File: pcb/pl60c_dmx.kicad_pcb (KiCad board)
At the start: 2 copper layers, 80 x 54 mm, 39 parts, among them J1 USB-C 16P, J2 XLR-5 female (DMX OUT), J3 DMX pigtail, J4 EXPANSION, J5 UART0, Q1 S8050, SW1 RESET, SW2 BOOT, SW3 USER, U1 ESP32-S3-WROOM-1-N16R8, U2 AMS1117-3.3, U3 SP3485EN, U4 USBLC6-2SC6

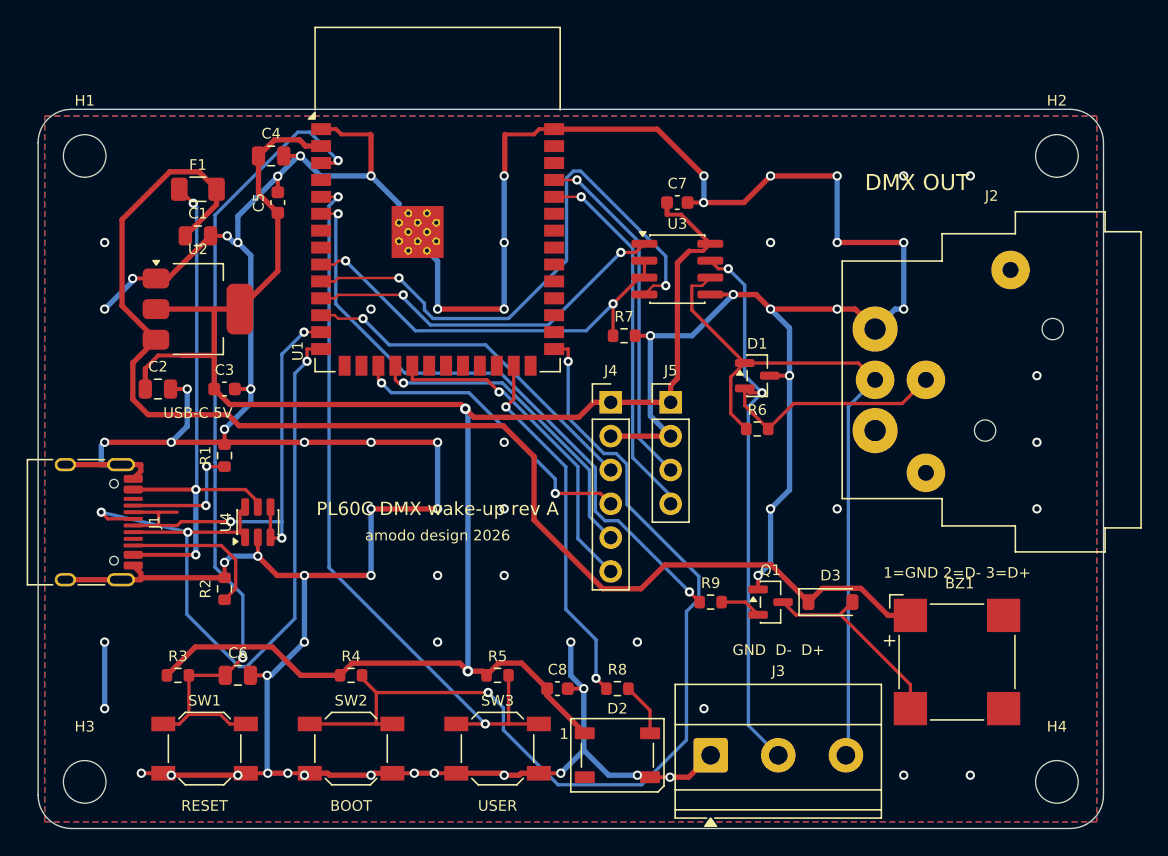
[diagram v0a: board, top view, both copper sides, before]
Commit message: auto: 2026-09-02 13:18:56
Co-Authored-By: Claude Fable 5.1 <noreply@anthropic.com>
Claude-Session: https://claude.ai/code/session_01WsrVZb94LwbHVAmBvsSTfn
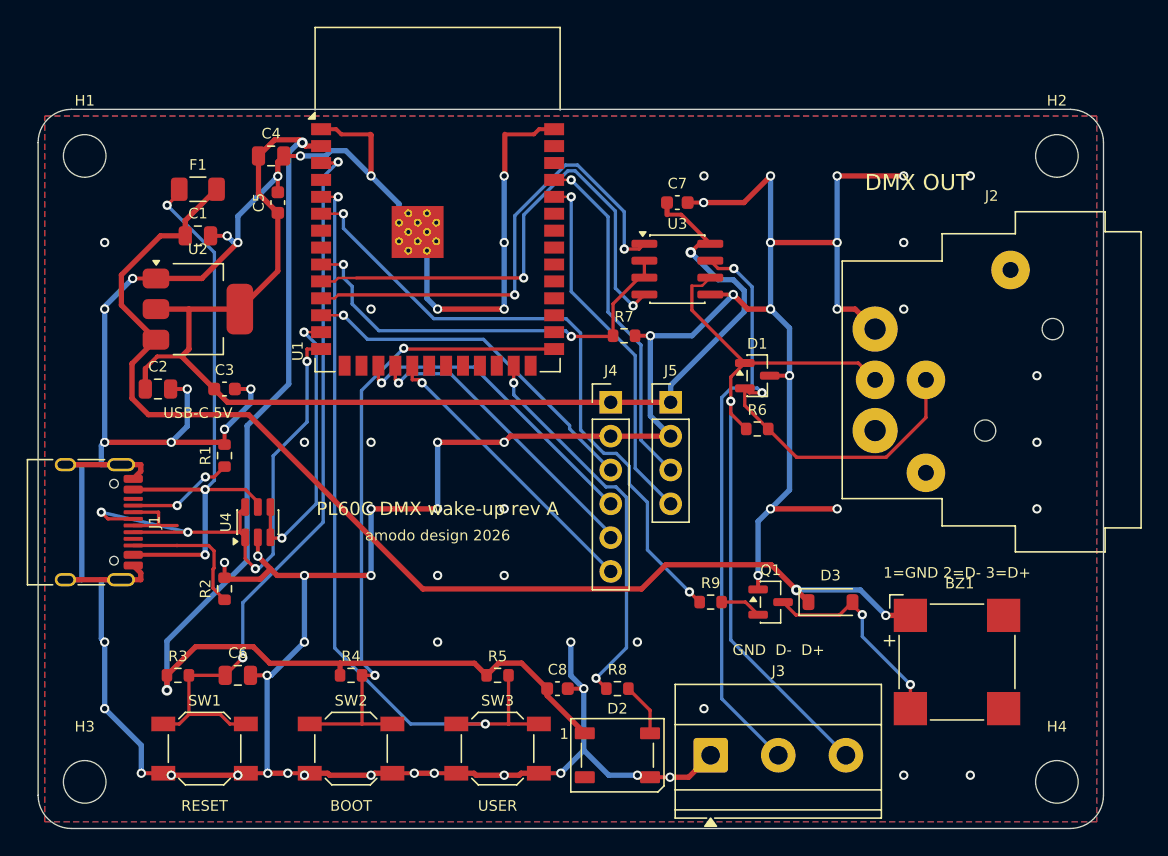
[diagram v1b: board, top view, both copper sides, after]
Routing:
- net +3V3: track 149.1 -> 177.8 mm, vias 2 -> 3
- net IO0_BOOT: track 74.2 -> 48.4 mm
- net USB_D+: track 59.0 -> 41.9 mm, vias 3 -> 4
- net +5V: track 99.1 -> 89.6 mm, vias 0 -> 2
- net USB_D-: track 36.2 -> 27.6 mm, vias 3 -> 2
- net DMX_RX: track 28.0 -> 36.3 mm
- net GND: track 360.9 -> 368.9 mm
- net EN: track 62.5 -> 55.8 mm
- net DMX_B: track 59.1 -> 65.7 mm
- net DMX_TX: track 42.5 -> 38.4 mm
- net EXP_IO11: track 25.1 -> 21.9 mm
- net BTN_USER: track 55.9 -> 58.8 mm
- net VBUS: track 42.8 -> 45.1 mm
- net LED_DATA: track 27.6 -> 29.5 mm
- net CC1: track 9.78 -> 8.08 mm
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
